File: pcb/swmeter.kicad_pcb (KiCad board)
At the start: 2 copper layers, 79.6 x 70 mm, 34 parts, among them J1 AudioPlug, J2 Conn_Coaxial, J3 Conn_01x03_Female, SW1 SW_SPDT, SW2 SW_SPDT, SW3 SW_DIP_x02, U1 LM3914N

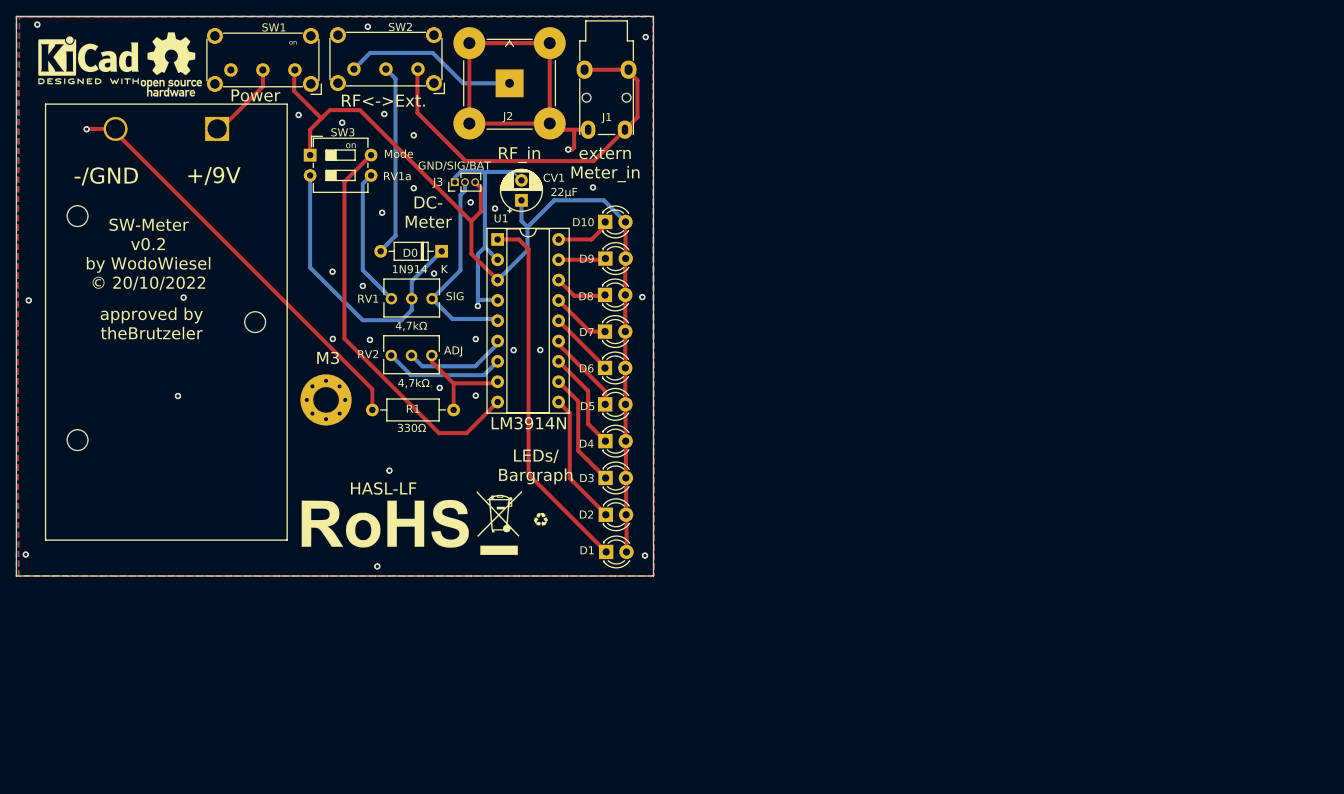
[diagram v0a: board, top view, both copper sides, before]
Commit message: update v0.4
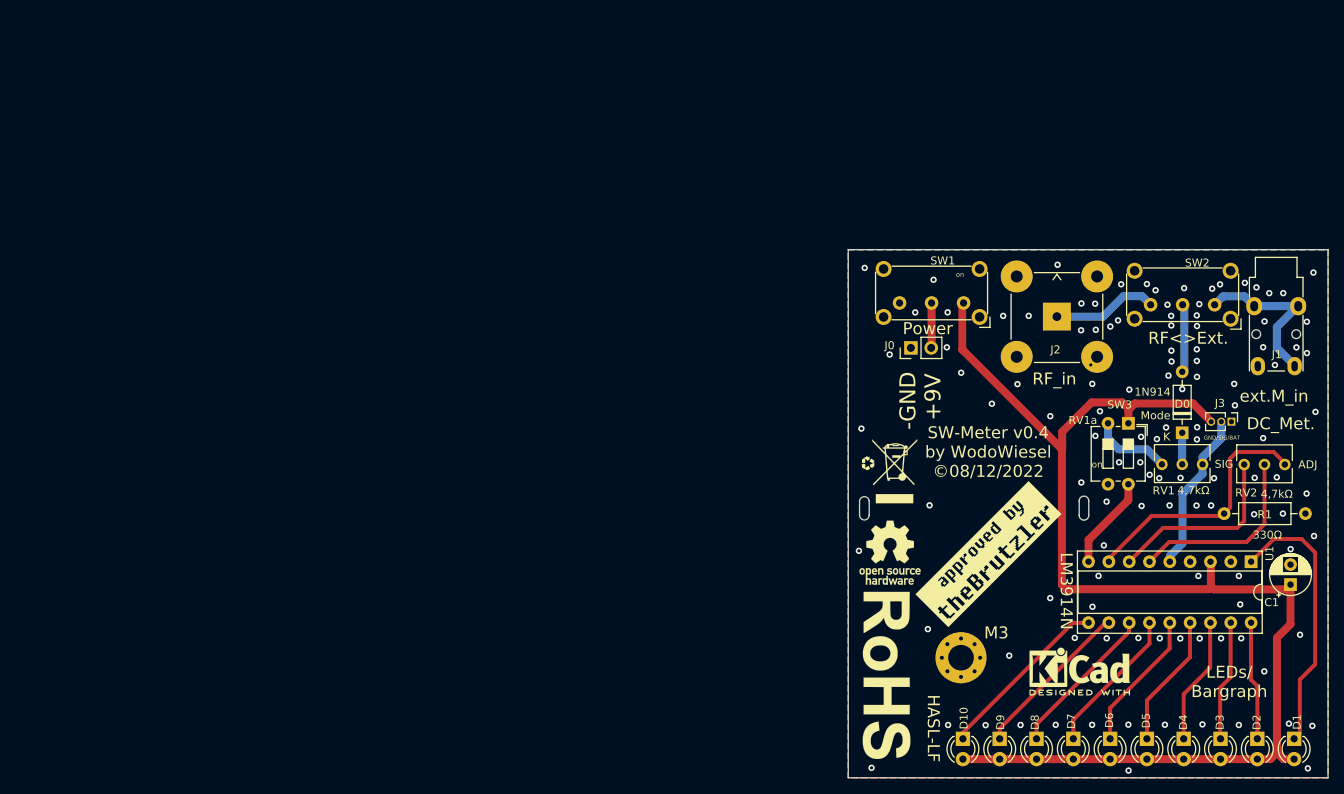
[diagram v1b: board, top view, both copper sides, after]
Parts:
- removed BT1: Battery_Cell, Battery:BatteryHolder_Eagle_12BH611-GR
- removed CV1: 22µF, Capacitor_THT:CP_Radial_D5.0mm_P2.50mm
- added C1: 22µF, Capacitor_THT:CP_Radial_D5.0mm_P2.50mm, F.Cu at (257.4, 126.3)
- added G1: LOGO, TheBrutzlers_Lib:approved_theBrutzler, F.Cu at (219.7, 122.5)
- added G11: LOGO, TheBrutzlers_Lib:approved_theBrutzler, B.Cu at (219.4, 122.5)
- added J0: Conn_01x02_Female, Connector_PinHeader_2.54mm:PinHeader_1x02_P2.54mm_Vertical, F.Cu at (210.0, 96.7)
- moved REF4 145.6 mm to (231.1, 137.1)
- moved REF44 145.3 mm to (230.8, 137.0)
- moved R1 117.4 mm to (259.3, 117.4), turned to 180 degrees
- moved REF3 108.6 mm to (207.4, 122.3)
- moved REF33 108.5 mm to (207.3, 122.3)
- moved SW3 107.6 mm to (237.2, 106.1), turned to -90 degrees
- moved RV2 107.5 mm to (251.6, 111.3)
- moved D2 104.0 mm to (253.3, 145.5), turned to -90 degrees
- moved SW2 103.8 mm to (247.9, 91.3)
- moved U1 102.4 mm to (252.5, 123.4), turned to -90 degrees
- moved J3 101.6 mm to (250.0, 105.9), turned to -90 degrees
- moved RV1 98.5 mm to (241.3, 111.2)
- moved D3 97.5 mm to (248.7, 145.5), turned to -90 degrees
- moved D0 95.3 mm to (243.9, 107.3), turned to 90 degrees
- moved D4 91.2 mm to (244.1, 145.5), turned to -90 degrees
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- renumbered D2 to D10, D10 to D2, D9 to D3, D8 to D4, D7 to D5, D5 to D7, D4 to D8, D3 to D9
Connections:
- SW3 pad 2: Net-(D0-Pad1) -> Net-(RV1-Pad1)
- SW3 pad 3: Net-(RV1-Pad1) -> GND
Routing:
- net GND: track 131.8 -> 0.59 mm, vias 33 -> 118
- net Net-(C1-Pad1): track 119.8 -> 175.7 mm
- net Net-(SW3-Pad4): track 50.0 -> 11.7 mm
- net Net-(D0-Pad1): track 36.5 -> 3.95 mm
- net Net-(J1-PadR): track 49.7 -> 20.6 mm
- net Net-(D0-Pad2): track 24.0 -> 8.28 mm
- net Net-(R1-Pad2): track 16.9 -> 32.3 mm
- net Net-(D1-Pad1): track 46.2 -> 34.3 mm
- net Net-(RV2-Pad2): track 12.8 -> 23.9 mm
- net Net-(D5-Pad1): track 7.41 -> 16.7 mm
- net Net-(D6-Pad1): track 8.30 -> 17.6 mm
- net Net-(D4-Pad1): track 6.66 -> 15.9 mm
- net Net-(D3-Pad1): track 5.91 -> 15.1 mm
- net Net-(RV2-Pad1): track 15.0 -> 23.7 mm
- net Net-(J2-Pad1): track 21.6 -> 13.2 mm
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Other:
- board size 79.6 x 70 mm -> 60 x 66 mm
- board text added: "+9V"
- board text added: "-GND"
- board text added: "C1"
- board text added: "DC_Met."
- board text added: "J0"
- board text added: "R<>Ext."
- board text added: "RF<>Ext."
- board text added: "SW-Meter v0.3 by WodoWiesel ©26/11/2022"
- board text added: "SW-Meter v0.4 by WodoWiesel ©08/12/2022"
- board text added: "ext.M_in"
- board text removed: "+/9V"
- board text removed: "-/GND"
- board text removed: "Battery"
- board text removed: "CV1"
- board text removed: "DC- Meter"
- board text removed: "R<->Ext."
- board text removed: "RF<->Ext."
- board text removed: "SW-Meter v0.2 by WodoWiesel © 20/10/2022"
- board text removed: "approved by theBrutzeler"
- board text removed: "extern Meter_in"
